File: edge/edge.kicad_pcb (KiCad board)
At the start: 2 copper layers, 47.5 x 47.7 mm, 4 parts

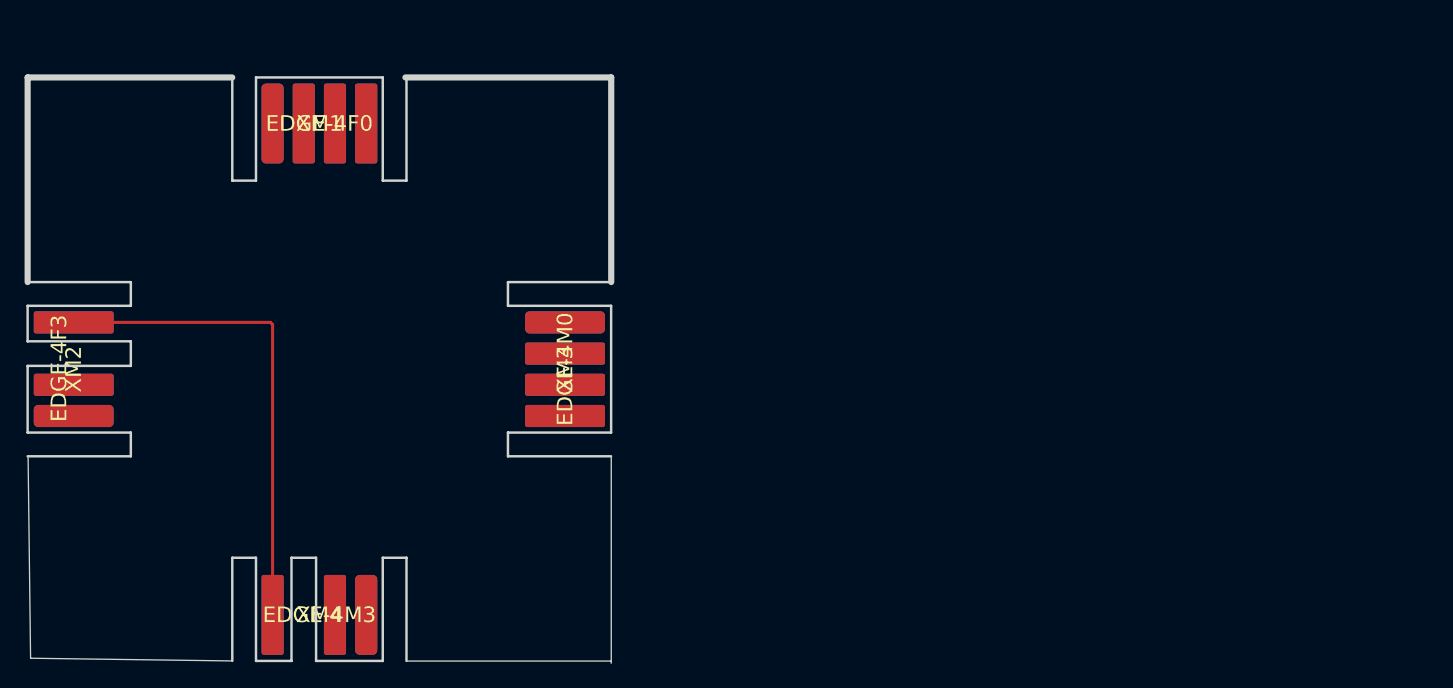
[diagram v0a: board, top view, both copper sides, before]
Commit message: fix generation script
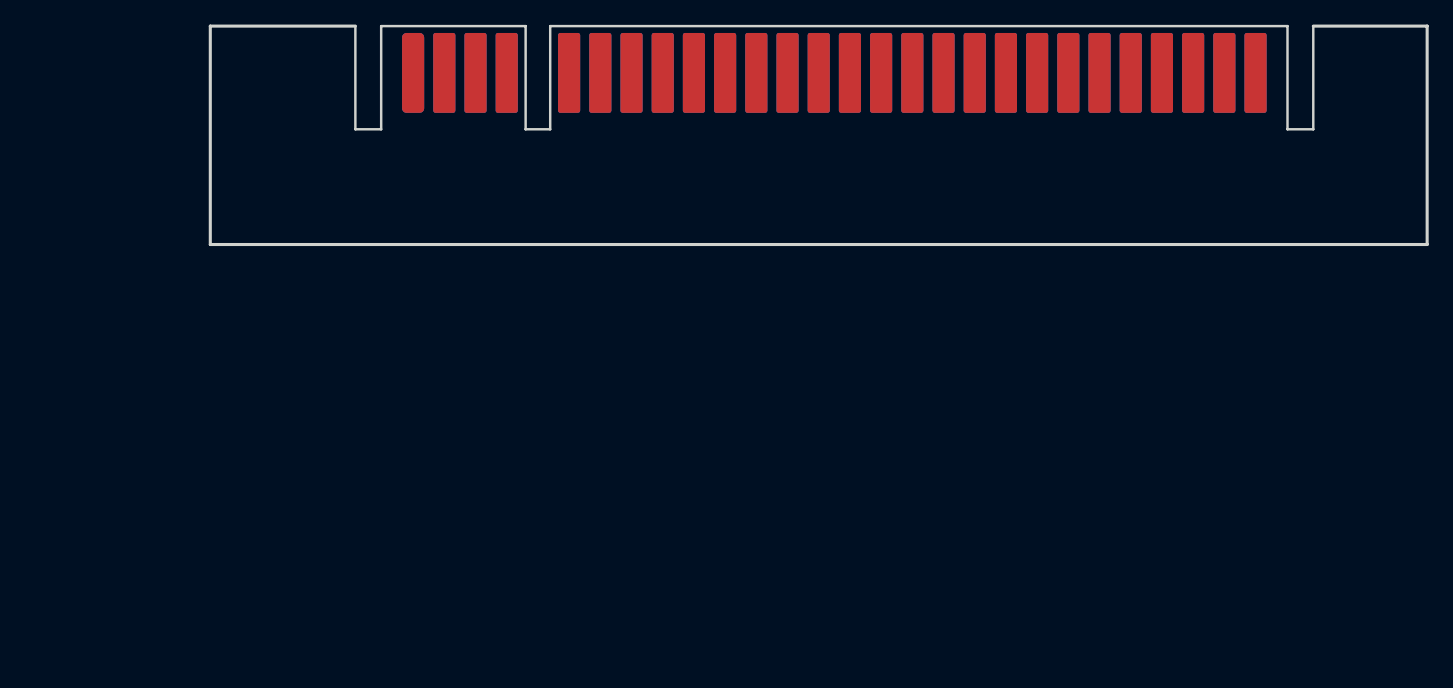
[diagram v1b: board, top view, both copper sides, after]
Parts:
- removed XM1: EDGE-4F0, edge:EDGE_4M0-2.54
- removed XM2: EDGE-4F3, edge:EDGE_4M3-2.54
- removed XM3: EDGE-4M0, edge:EDGE_4M0-2.54
- removed XM4: EDGE-4M3, edge:EDGE_4M3-2.54
- added ?: , edge:EDGE_28M5-2.54, F.Cu at (121.9, 55.9)
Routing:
- net /MD3: track 39.9 -> 0.00 mm
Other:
- board size 47.5 x 47.7 mm -> 99.1 x 17.8 mm
- net class Default removed

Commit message: test pcb
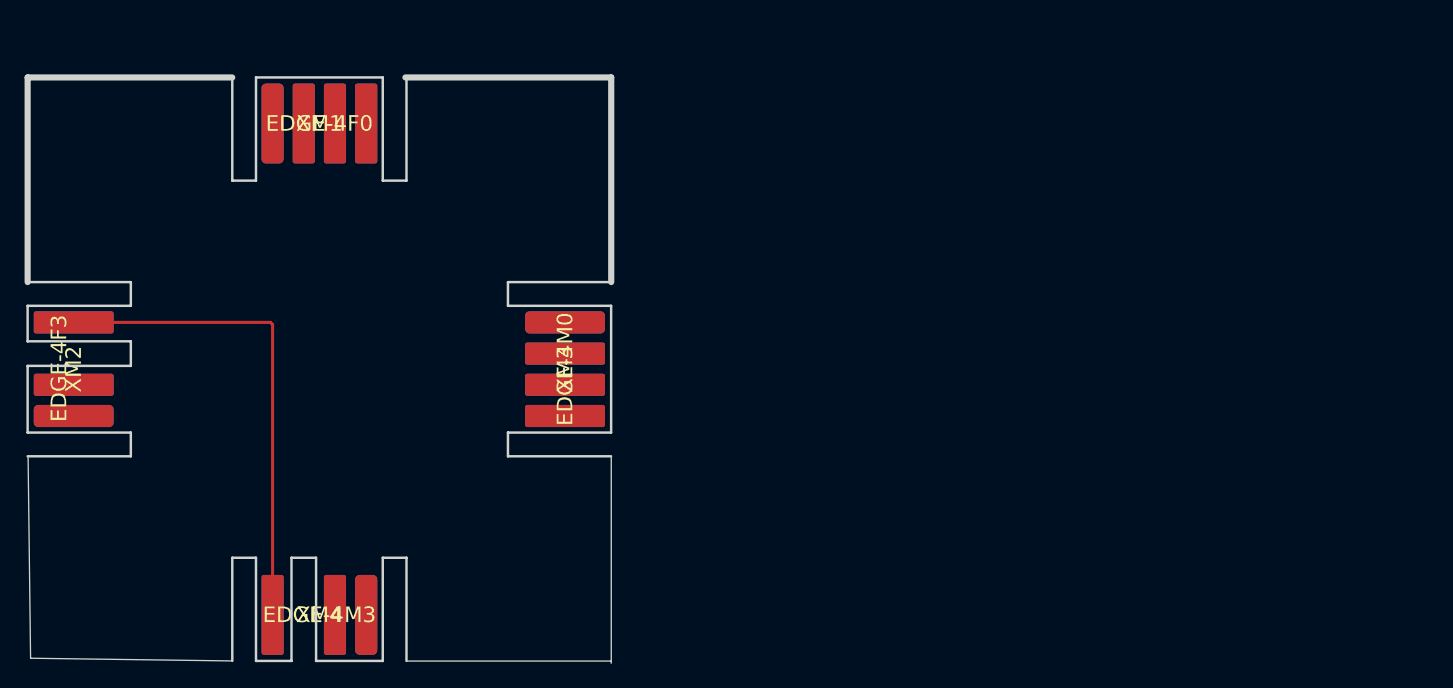
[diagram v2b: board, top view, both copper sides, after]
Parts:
- removed ?: , edge:EDGE_28M5-2.54
- added XM1: EDGE-4F0, edge:EDGE_4M0-2.54, F.Cu at (80.0, 60.0)
- added XM2: EDGE-4F3, edge:EDGE_4M3-2.54, F.Cu at (60.0, 80.0)
- added XM3: EDGE-4M0, edge:EDGE_4M0-2.54, F.Cu at (100.0, 80.0)
- added XM4: EDGE-4M3, edge:EDGE_4M3-2.54, F.Cu at (80.0, 100.0)
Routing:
- net /MD3: track 0.00 -> 39.9 mm
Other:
- board size 99.1 x 17.8 mm -> 47.5 x 47.7 mm
